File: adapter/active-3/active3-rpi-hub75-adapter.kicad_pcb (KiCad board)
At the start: 2 copper layers, 83 x 35.5 mm, 24 parts, among them P1 CONN_02X20, P2 +5V, P20 CONN_01X01, P21 CONN_01X01, P3 RxD, P4 GND, P5 GND, P6 CONN_01X02, P7 CONN_02X01, P8 CONN_01X02, U1 74HCT245, U2 74HCT245, U3 74HCT245

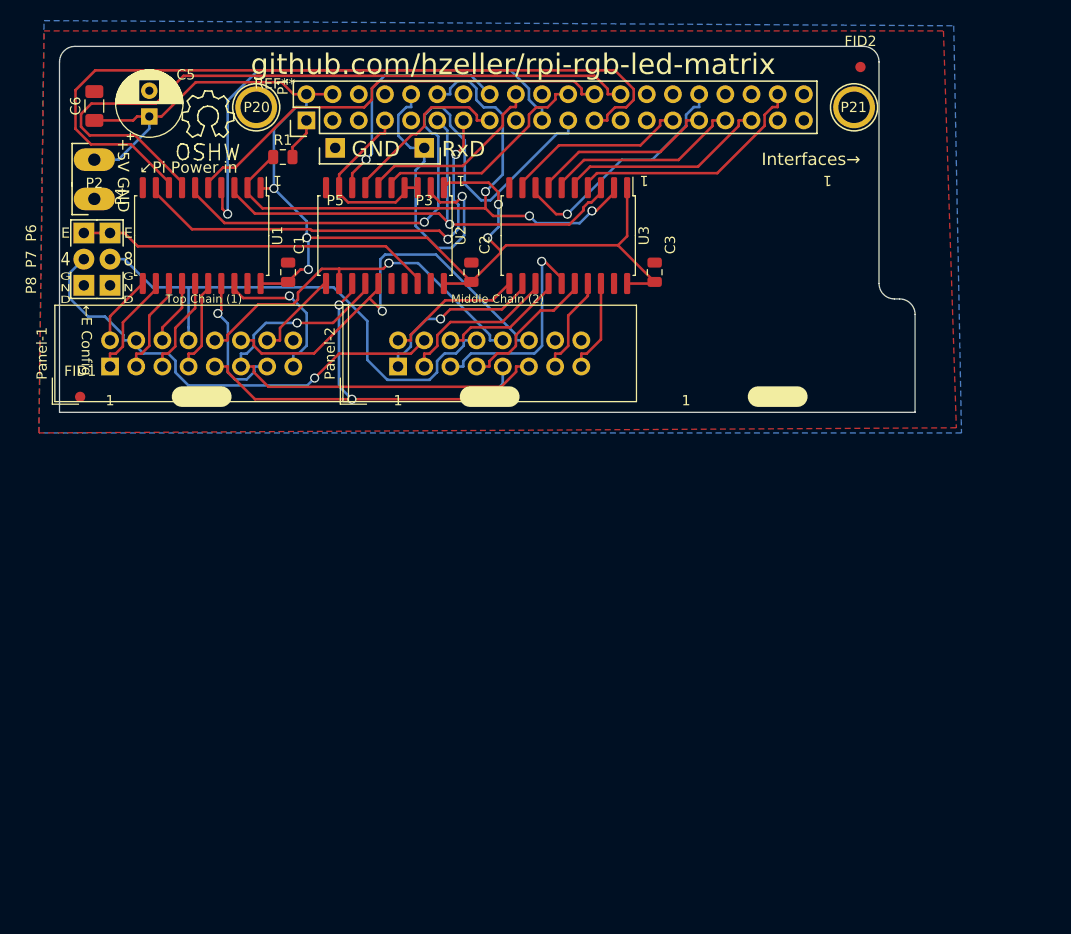
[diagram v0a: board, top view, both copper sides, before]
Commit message: newer schematics
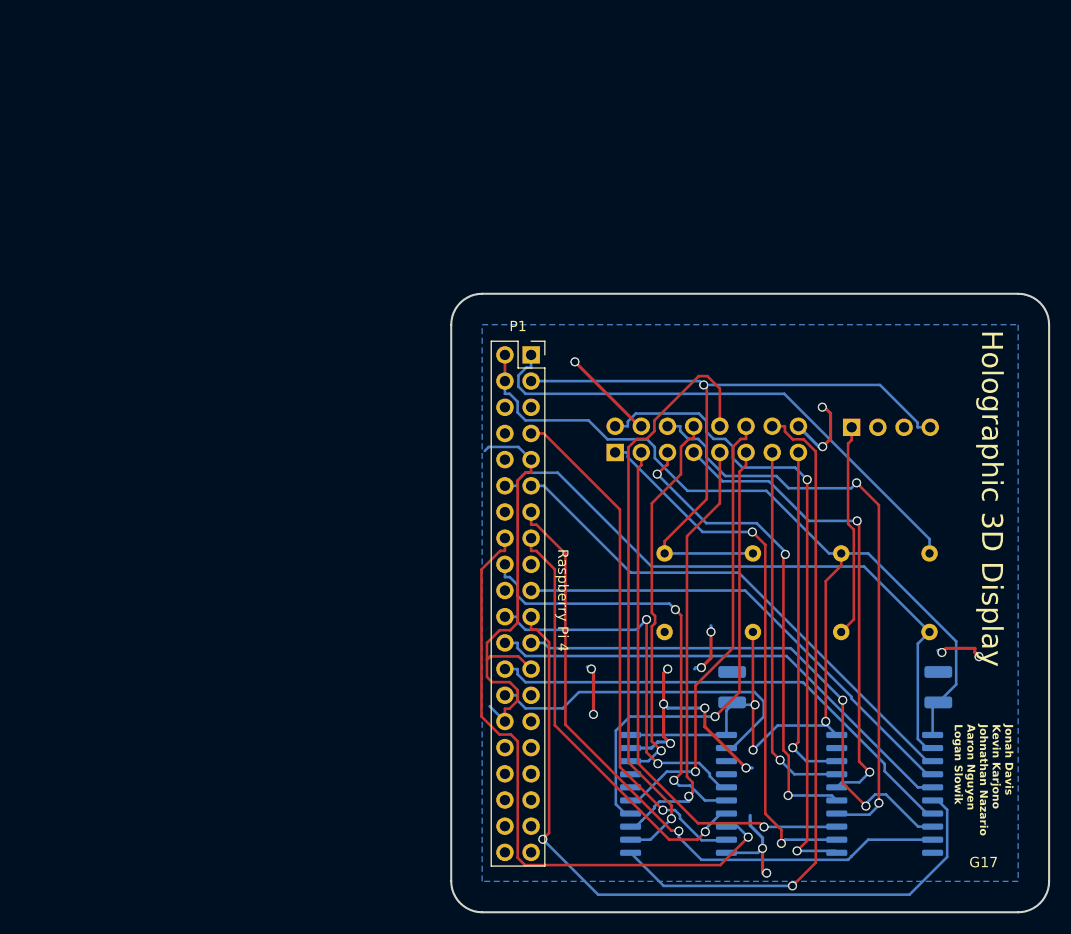
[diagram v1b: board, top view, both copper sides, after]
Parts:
- removed C3: 100n, Capacitor_SMD:C_0805_2012Metric
- removed C5: 22u, Capacitor_THT:CP_Radial_D6.3mm_P2.50mm
- removed C6: 22u, Capacitor_SMD:C_1206_3216Metric
- removed FID1: BottomLeft, Fiducial:Fiducial_1mm_Dia_2.54mm_Outer_CopperTop
- removed FID2: TopRight, Fiducial:Fiducial_1mm_Dia_2.54mm_Outer_CopperTop
- removed P2: +5V, Pin_Headers:Pin_Header_Straight_1x01
- removed P20, P21: CONN_01X01, Connect:1pin
- removed P3: RxD, Pin_Headers:Pin_Header_Straight_1x01
- removed P4, P5: GND, Pin_Headers:Pin_Header_Straight_1x01
- removed P6, P8: CONN_01X02, Pin_Headers:Pin_Header_Straight_1x02
- removed P7: CONN_02X01, Pin_Headers:Pin_Header_Straight_1x02
- removed Panel-2: CONN_02X08, Connector_IDC:IDC-Header_2x08_P2.54mm_Vertical
- removed REF**: Symbol_OSHW-Logo_SilkScreen, Symbols:Symbol_OSHW-Logo_SilkScreen
- removed U3: 74HCT245, Package_SO:SOIC-20W_7.5x12.8mm_P1.27mm
- added J1: IR_Sensor_Socket, Connector_PinSocket_2.54mm:PinSocket_1x04_P2.54mm_Horizontal, B.Cu at (160.8, 73.0)
- added R5: 10k, Resistor_THT:R_Axial_DIN0207_L6.3mm_D2.5mm_P7.62mm_Horizontal, B.Cu at (151.3, 92.8)
- added R6: 470, Resistor_THT:R_Axial_DIN0207_L6.3mm_D2.5mm_P7.62mm_Horizontal, B.Cu at (159.8, 92.8)
- added R7: 20k, Resistor_THT:R_Axial_DIN0207_L6.3mm_D2.5mm_P7.62mm_Horizontal, B.Cu at (142.7, 92.8)
- C1, C2: footprint Capacitor_SMD:C_0805_2012Metric -> Capacitor_SMD:C_1210_3225Metric; moved to B.Cu
- P1: footprint Pin_Headers:Pin_Header_Straight_2x20 -> Connector_PinSocket_2.54mm:PinSocket_2x20_P2.54mm_Vertical
- Panel-1: footprint Connector_IDC:IDC-Header_2x08_P2.54mm_Vertical -> Connector_PinSocket_2.54mm:PinSocket_2x08_P2.54mm_Horizontal; moved to B.Cu
- R1: footprint Resistor_SMD:R_0805_2012Metric -> Resistor_THT:R_Axial_DIN0207_L6.3mm_D2.5mm_P7.62mm_Horizontal; moved to B.Cu
- U1, U2: moved to B.Cu
- moved U1 85.6 mm to (164.1, 108.5), turned to 180 degrees
- moved R1 77.8 mm to (168.4, 92.8), turned to 90 degrees
- moved C1 74.8 mm to (169.2, 98.2)
- moved U2 61.2 mm to (144.1, 108.5), turned to 180 degrees
- moved Panel-1 49.7 mm to (137.9, 75.4), turned to -90 degrees
- moved C2 47.5 mm to (149.2, 98.2)
- moved P1 31.5 mm to (129.8, 65.9), turned to 0 degrees
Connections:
- P1 pad 10: row_E -> UART_RX
- P1 pad 17: unconnected-(P1-Pin_17-Pad17) -> /3v3
- P1 pad 28: unconnected-(P1-Pin_28-Pad28) -> row_E
- P1 pad 3: unconnected-(P1-Pin_3-Pad3) -> spin_sync
- P1 pad 30: unconnected-(P1-Pin_30-Pad30) -> GND
- P1 pad 8: unconnected-(P1-Pin_8-Pad8) -> UART_TX
- P1 pad 9: unconnected-(P1-Pin_9-Pad9) -> GND
- Panel-1 pad 4: Sel-Pin4 -> GND
- Panel-1 pad 8: Sel-Pin8 -> row_E_buff
- U2 pad 16: strobe_buff_1 -> unconnected-(U2-B2-Pad16)
- U2 pad 17: strobe_buff_2 -> unconnected-(U2-B1-Pad17)
- U2 pad 18: Net-(P6-Pin_1) -> row_E_buff
- U2 pad 3: strobe -> unconnected-(U2-A1-Pad3)
- U2 pad 4: strobe -> unconnected-(U2-A2-Pad4)
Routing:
- net GND: track 0.00 -> 109.5 mm, vias 0 -> 16
- net spin_sync: track 0.00 -> 67.6 mm, vias 0 -> 1
- net strobe_buff_0: track 8.70 -> 65.6 mm, vias 0 -> 1
- net p0_g1_buff: track 6.83 -> 63.7 mm, vias 0 -> 2
- net p0_g2_buff: track 6.30 -> 58.6 mm, vias 0 -> 2
- net Sel-Pin8: track 50.3 -> 0.00 mm
- net Net-(P1-Pin_1): track 4.11 -> 51.3 mm
- net Sel-Pin4: track 45.6 -> 0.00 mm, vias 1 -> 0
- net p0_r1_buff: track 10.2 -> 53.7 mm, vias 0 -> 2
- net p0_b1_buff: track 9.67 -> 52.1 mm, vias 0 -> 1
- net p0_b2_buff: track 9.14 -> 47.3 mm, vias 0 -> 2
- net row_B: track 23.1 -> 60.6 mm
- net row_E_buff: track 0.00 -> 37.5 mm, vias 0 -> 1
- net p0_r2_buff: track 9.68 -> 47.0 mm, vias 0 -> 3
- net Net-(P6-Pin_1): track 34.7 -> 0.00 mm
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- removed copper zone on F.Cu, net GND
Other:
- board size 83 x 35.5 mm -> 58 x 60 mm
- board text added: "10k"
- board text added: "20k"
- board text added: "470"
- board text added: "Color Data"
- board text added: "G17"
- board text added: "Holographic 3D Display"
- board text added: "IR Sensor"
- board text added: "Jonah Davis Kevin Karjono Johnathan Nazario Aaron Nguyen Logan Slowik"
- board text added: "Matrix"
- board text added: "Raspberry Pi 4"
- board text added: "Row Data"
- board text removed: "%%gitversion%%"
- board text removed: "+5V GND"
- board text removed: "1"
- board text removed: "4"
- board text removed: "8"
- board text removed: "E"
- board text removed: "G N D"
- board text removed: "Interfaces→"
- board text removed: "Middle Chain (2)"
- board text removed: "Top Chain (1)"
- board text removed: "github.com/hzeller/rpi-rgb-led-matrix"
- board text removed: "←E Config"
- board text removed: "↙Pi Power in"
